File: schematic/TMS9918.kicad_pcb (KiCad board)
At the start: 2 copper layers, 74.9 x 81.3 mm, 21 parts, among them J1 Bus, J2 Video out, J3 Power, Q1 2N4401, U1 TMS9918A, U2 HM62256BLP, U3 74HCT574, U4 74HCT574, U5 74HCT574, U6 74HCT04, Y1 10.738635MHz

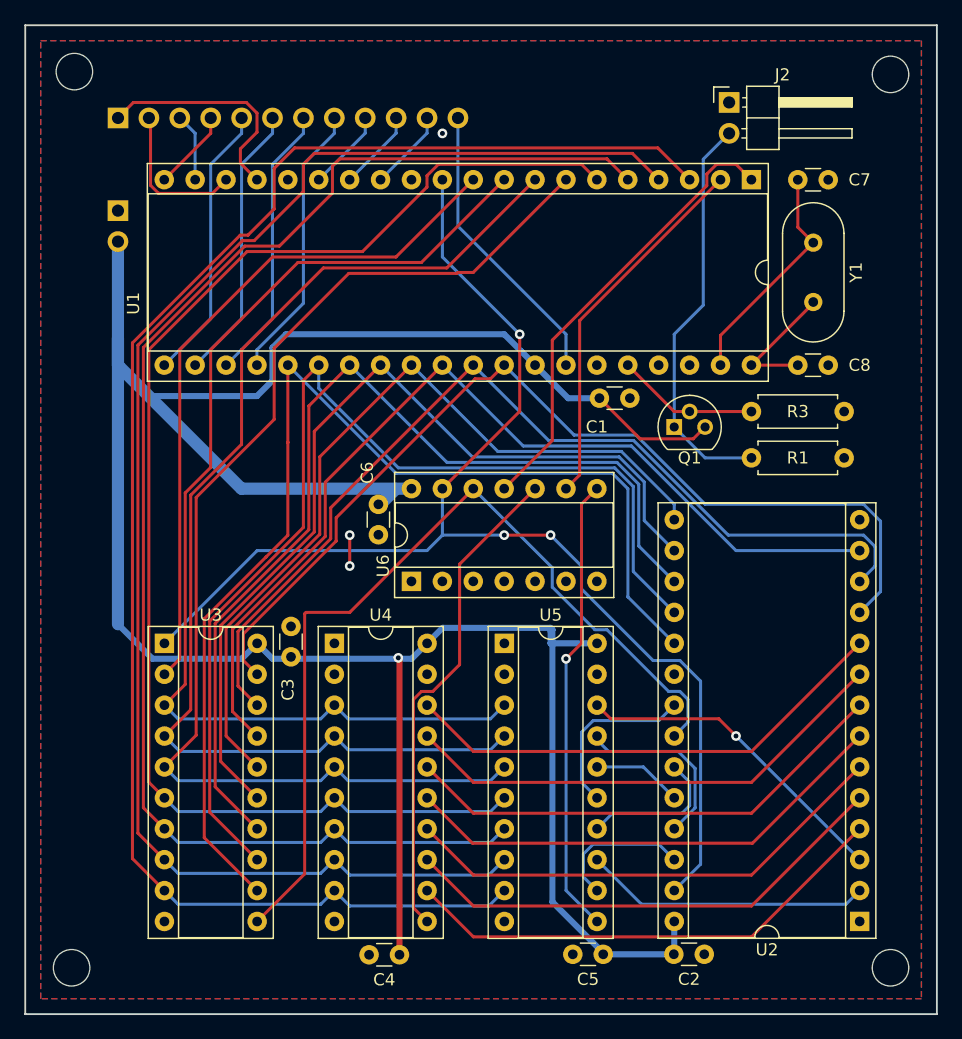
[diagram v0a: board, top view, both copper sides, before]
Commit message: V1.1
Various improvements
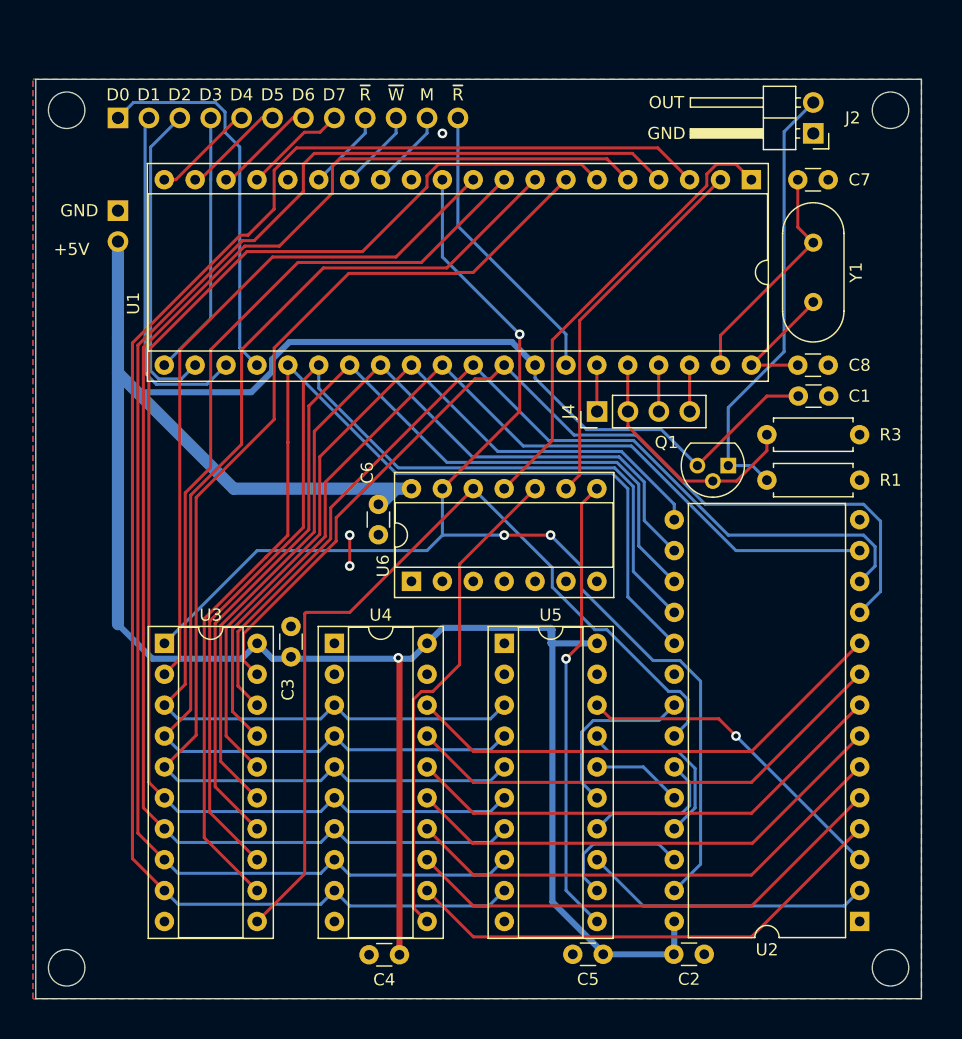
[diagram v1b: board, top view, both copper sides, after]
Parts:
- added J4: Conn_01x04_Female, Connector_PinHeader_2.54mm:PinHeader_1x04_P2.54mm_Vertical, F.Cu at (90.2, 87.6)
- C7, C8: value 16pf -> 22pf
- Q1: value 2N4401 -> Q_NPN_EBC
- R1: value 75 -> 1k
- U2: footprint Package_DIP:DIP-28_W15.24mm_Socket -> Package_DIP:DIP-28_W15.24mm
- moved C1 16.3 mm to (106.7, 86.4)
- moved J2 7.37 mm to (108.0, 64.8), turned to 180 degrees
- moved Q1 5.46 mm to (101.0, 92.1), turned to 180 degrees
- moved R3 2.29 mm to (104.1, 89.5)
- moved R1 2.23 mm to (104.1, 93.3)
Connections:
- net /R~{W} renamed R~{W}
- net /VD0 renamed VD0
- net /VD1 renamed VD1
- net /VD2 renamed VD2
- net /VD3 renamed VD3
- net /VD4 renamed VD4
- net /VD5 renamed VD5
- net /VD6 renamed VD6
- net /VD7 renamed VD7
- net /~{R}W renamed ~{R}W
- net Net-(Q1-Pad2) renamed /vid
- U1 pad 16: /~{INT} -> unconnected-(U1-Pad16)
- U1 pad 17: /D0 -> /D7
- U1 pad 18: /D1 -> /D6
- U1 pad 19: /D2 -> /D5
- U1 pad 20: /D3 -> /D4
- U1 pad 21: /D4 -> /D3
- U1 pad 22: /D5 -> /D2
- U1 pad 23: /D6 -> /D1
- U1 pad 24: /D7 -> /D0
- U1 pad 35: /EXTVDP -> /EXT
- U1 pad 37: /GROMCLK -> Net-(U1-Pad37)
- U1 pad 38: /CPUCLK -> Net-(U1-Pad38)
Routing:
- net /D2: track 5.60 -> 26.2 mm
- net /D1: track 12.5 -> 28.8 mm
- net /D3: track 6.65 -> 21.9 mm
- net /D7: track 22.9 -> 8.46 mm
- net /D6: track 22.9 -> 8.46 mm
- net /D5: track 22.9 -> 8.46 mm
- net /D4: track 22.9 -> 8.46 mm
- net /D0: track 18.9 -> 31.5 mm
- net /vid: track 11.7 -> 20.7 mm
- net Net-(U1-Pad38): track 0.00 -> 3.82 mm
- net Net-(U1-Pad37): track 0.00 -> 3.82 mm
- net /EXT: track 0.00 -> 3.82 mm
- net Net-(J2-Pad2): track 33.4 -> 36.4 mm
- net VCC: track 229.4 -> 231.9 mm
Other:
- board size 74.9 x 81.3 mm -> 72.8 x 75.6 mm
- board text added: "+5V"
- board text added: "D0"
- board text added: "D1"
- board text added: "D2"
- board text added: "D3"
- board text added: "D4"
- board text added: "D5"
- board text added: "D6"
- board text added: "D7"
- board text added: "GND"
- board text added: "M"
- board text added: "OUT"
- board text added: "~{R}"
- board text added: "~{W}"
